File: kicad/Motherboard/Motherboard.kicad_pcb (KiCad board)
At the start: 2 copper layers, 72.6 x 54.1 mm, 71 parts, among them J1 USB_C_Receptacle_USB2.0, J10 Conn_01x08_Pin, J11 Conn_01x08_Pin, J12 Conn_01x08_Pin, J13 Conn_01x08_Pin, J2 Conn_01x02_Pin, J3 Conn_01x04_Pin, J4 Conn_01x04_Pin, J5 Conn_01x02_Pin, J6 Conn_01x08_Pin, J7 Conn_01x08_Pin, J8 Conn_01x08_Pin, J9 Conn_01x08_Pin, Q1 DMN3404L, SW1 Reset, SW2 Boot, U1 ESP32-S2-SOLO, U2 LD1117S33TR_SOT223, U3 TCA9535RTWR, U4 TCA9535RTWR, U5 TCA9535RTWR, U6 TCA9535RTWR, U7 TMC2208-LA, U8 TMC2208-LA, U9 LM2575-5.0BT

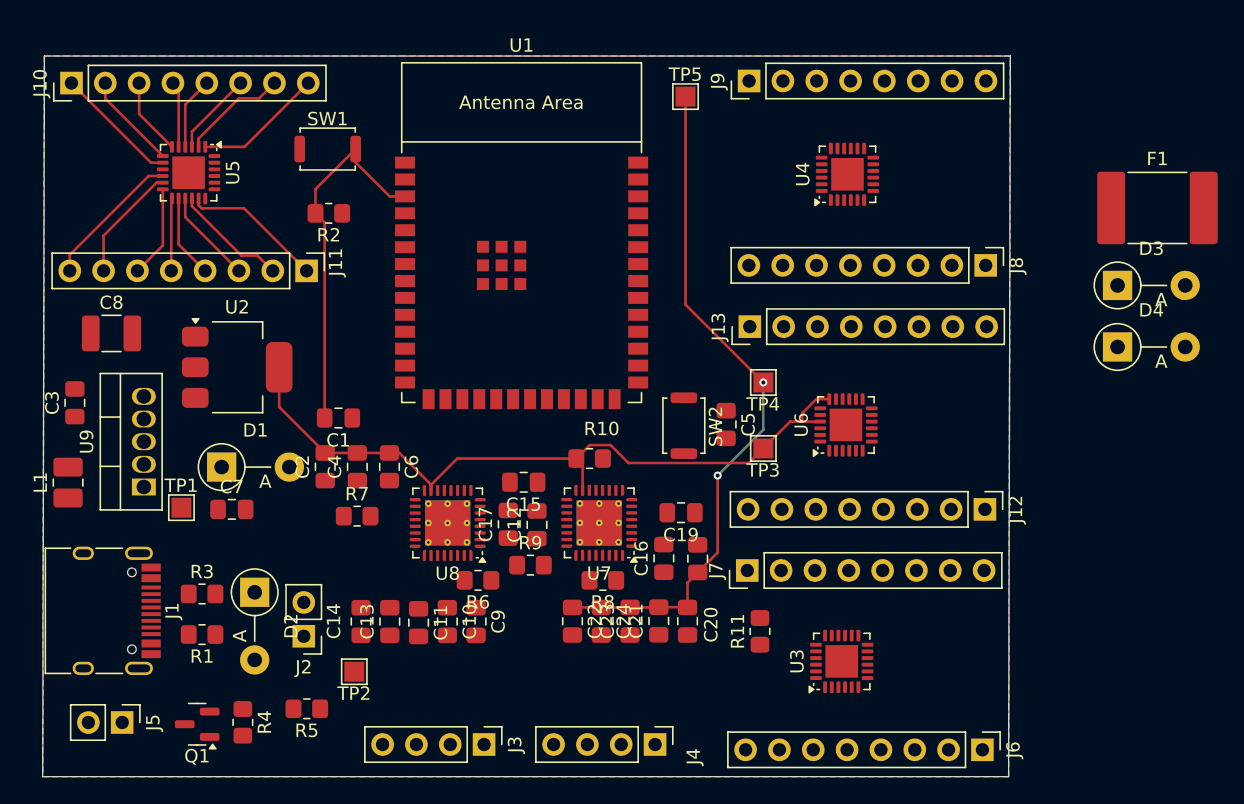
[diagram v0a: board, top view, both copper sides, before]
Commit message: finish pls sia
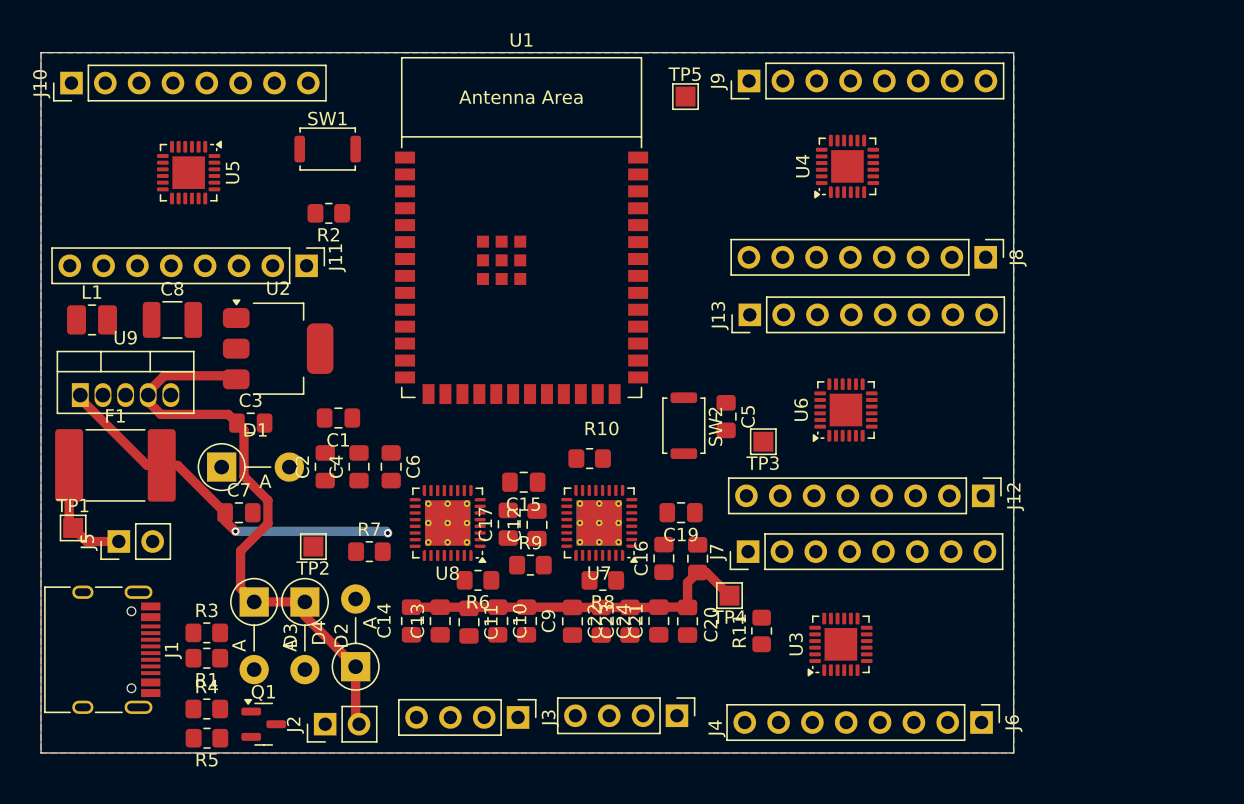
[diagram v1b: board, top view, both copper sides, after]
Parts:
- moved F1 80.6 mm to (89.5, 108.8)
- moved D3 69.0 mm to (99.9, 119.1), turned to -90 degrees
- moved D4 62.0 mm to (107.6, 124.0), turned to 90 degrees
- moved TP4 16.2 mm to (135.6, 118.6)
- moved J5 13.6 mm to (89.8, 114.6), turned to 90 degrees
- moved C3 13.3 mm to (99.7, 105.7), turned to 0 degrees
- moved L1 12.3 mm to (87.8, 97.9), turned to 0 degrees
- moved TP2 9.88 mm to (104.4, 114.9)
- moved U9 8.39 mm to (86.9, 103.6), turned to 0 degrees
- moved TP1 8.27 mm to (86.4, 113.5)
- moved R5 7.81 mm to (96.4, 129.3)
- moved J2 6.80 mm to (105.3, 128.3), turned to 90 degrees
- moved Q1 4.99 mm to (100.7, 128.3), turned to 0 degrees
- moved C8 4.68 mm to (93.8, 97.9)
- moved D2 3.84 mm to (103.8, 119.1)
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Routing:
- net +3.3V: track 55.6 -> 0.00 mm
- net +5V: track 0.00 -> 45.6 mm
- net Net-(U1-EN): track 27.5 -> 0.00 mm
- net Net-(J11-Pin_1): track 10.7 -> 0.00 mm
- net Net-(J11-Pin_8): track 10.6 -> 0.00 mm
- net Net-(J10-Pin_8): track 9.72 -> 0.00 mm
- net Net-(J10-Pin_1): track 9.33 -> 0.00 mm
- net Net-(J11-Pin_7): track 8.74 -> 0.00 mm
- net Net-(J5-Pin_1): track 0.00 -> 8.67 mm
- net Net-(J11-Pin_2): track 8.65 -> 0.00 mm
- net Net-(J10-Pin_7): track 8.04 -> 0.00 mm
- net Net-(J10-Pin_2): track 7.27 -> 0.00 mm
- net Net-(J11-Pin_3): track 7.10 -> 0.00 mm
- net Net-(J11-Pin_6): track 6.91 -> 0.00 mm
- net Net-(J10-Pin_6): track 6.30 -> 0.00 mm
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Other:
- board size 72.6 x 54.1 mm -> 73 x 52.6 mm
